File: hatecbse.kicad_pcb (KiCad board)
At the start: 2 copper layers, 79 x 88.8 mm, 20 parts, among them J1 Screw_Terminal_01x06, J2 Screw_Terminal_01x06, J3 Barrel_Jack_MountingPin, J4 Conn_01x04_Socket, J5 Conn_01x03, J6 Conn_01x02_Pin, J7 Conn_01x02_Pin, J8 Conn_01x04_Pin, U1 TMC2209_SILENTSTEPSTICK, U2 TMC2209_SILENTSTEPSTICK

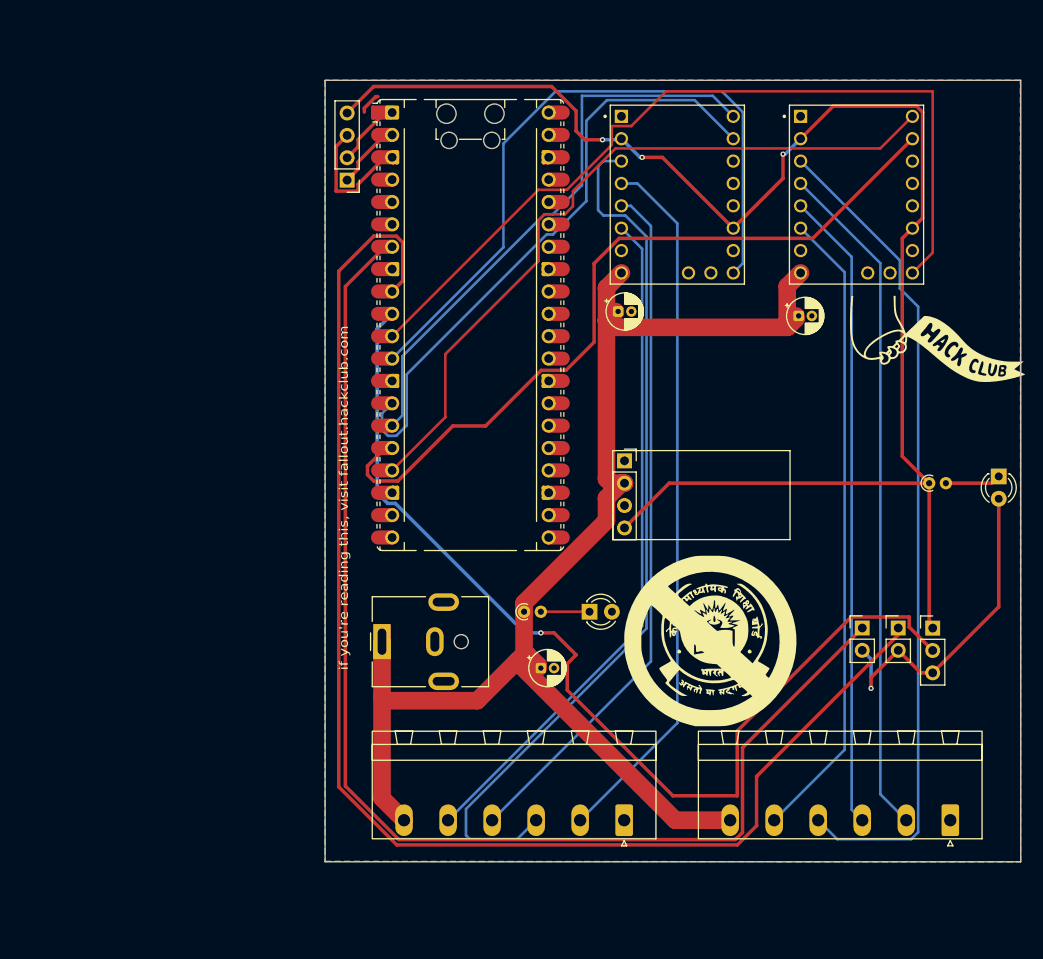
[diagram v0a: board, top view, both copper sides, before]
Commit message: diddy
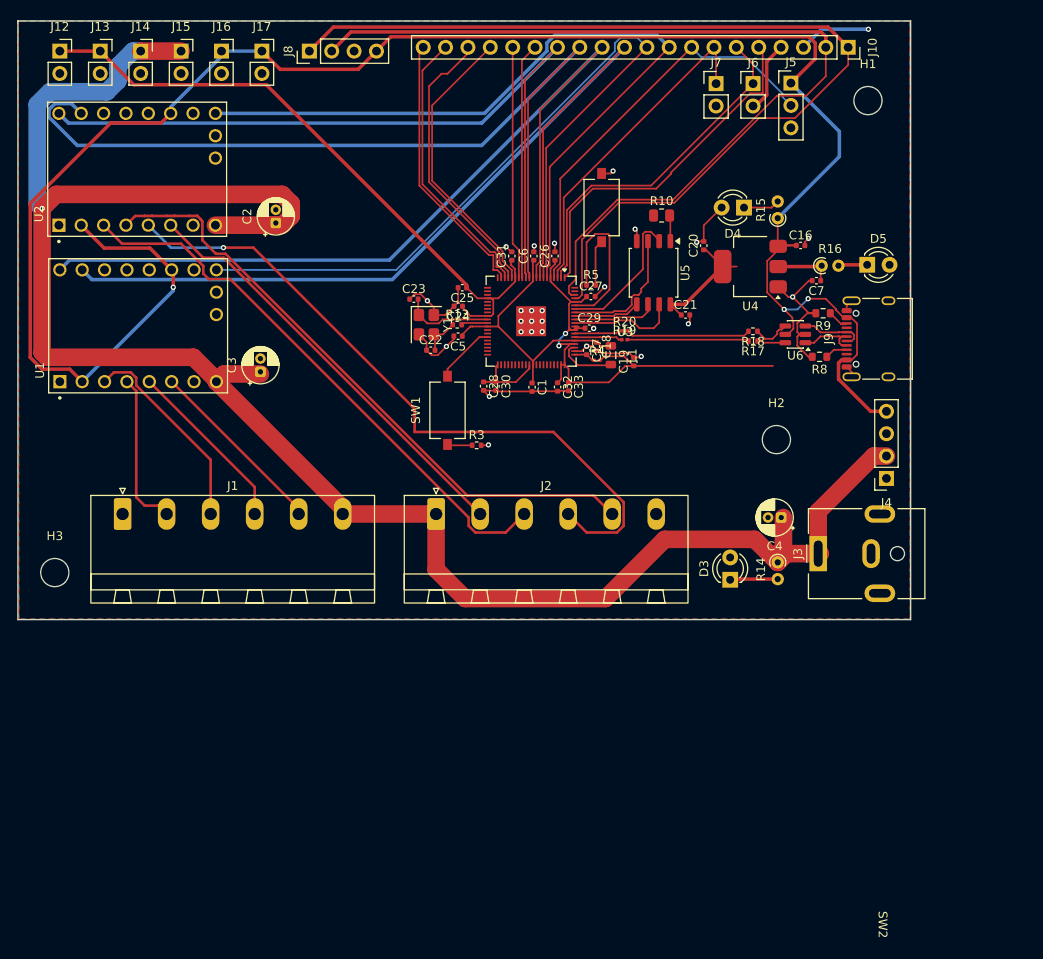
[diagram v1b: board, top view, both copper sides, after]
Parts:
- removed A1: RaspberryPi_Pico, Module:RaspberryPi_Pico_Common_Unspecified
- removed D1, D2: LED, LED_THT:LED_D3.0mm
- removed G*** (x2): LOGO, LOGO
- removed R1: 1.2k, Resistor_THT:R_Axial_DIN0204_L3.6mm_D1.6mm_P1.90mm_Vertical
- removed R2: 500, Resistor_THT:R_Axial_DIN0204_L3.6mm_D1.6mm_P1.90mm_Vertical
- added C1: 100 n, Capacitor_SMD:C_0402_1005Metric, F.Cu at (131.5, 94.6)
- added C16: 10 u, Capacitor_SMD:C_0402_1005Metric, F.Cu at (162.0, 78.5)
- added C17: 4.7 u, Capacitor_SMD:C_0402_1005Metric, F.Cu at (137.7, 90.4)
- added C18: 4.7 u, Capacitor_SMD:C_0402_1005Metric, F.Cu at (138.8, 90.0)
- added C19: 4.7 u, Capacitor_SMD:C_0402_1005Metric, F.Cu at (143.1, 91.7)
- added C20: 10 u, Capacitor_SMD:C_0402_1005Metric, F.Cu at (151.0, 78.5)
- added C21: 100 n, Capacitor_SMD:C_0402_1005Metric, F.Cu at (148.9, 86.4)
- added C22: 15 p, Capacitor_SMD:C_0402_1005Metric, F.Cu at (120.0, 90.4)
- added C23: 15 p, Capacitor_SMD:C_0402_1005Metric, F.Cu at (118.1, 84.6)
- added C24: 100 n, Capacitor_SMD:C_0402_1005Metric, F.Cu at (123.1, 85.4)
- added C25: 100 n, Capacitor_SMD:C_0402_1005Metric, F.Cu at (123.6, 83.3)
- added C26: 100 n, Capacitor_SMD:C_0402_1005Metric, F.Cu at (134.1, 79.7)
- added C27: 100 n, Capacitor_SMD:C_0402_1005Metric, F.Cu at (138.2, 84.3)
- added C28: 100 n, Capacitor_SMD:C_0402_1005Metric, F.Cu at (126.0, 94.5)
- added C29: 100 n, Capacitor_SMD:C_0402_1005Metric, F.Cu at (138.0, 87.9)
- added C30: 100 n, Capacitor_SMD:C_0402_1005Metric, F.Cu at (127.4, 94.5)
- added C31: 100 n, Capacitor_SMD:C_0402_1005Metric, F.Cu at (129.2, 79.7)
- added C32: 100 n, Capacitor_SMD:C_0402_1005Metric, F.Cu at (134.4, 94.6)
- added C33: 100 n, Capacitor_SMD:C_0402_1005Metric, F.Cu at (135.7, 94.5)
- added C5: 4.7 u, Capacitor_SMD:C_0402_1005Metric, F.Cu at (123.1, 88.8)
- added C6: 100 n, Capacitor_SMD:C_0402_1005Metric, F.Cu at (131.7, 79.7)
- added C7: 10 uF, Capacitor_SMD:C_0402_1005Metric, F.Cu at (163.8, 82.5)
- added D3: LED, LED_THT:LED_D3.0mm, F.Cu at (154.0, 116.5)
- added D4: LED, LED_THT:LED_D3.0mm, F.Cu at (155.6, 74.2)
- added D5: LED, LED_THT:LED_D3.0mm, F.Cu at (169.6, 80.7)
- added H1: MountingHole, MountingHole:MountingHole_3.2mm_M3, F.Cu at (169.7, 62.0)
- added H2: MountingHole, MountingHole:MountingHole_3.2mm_M3, F.Cu at (159.2, 100.5)
- added H3: MountingHole, MountingHole:MountingHole_3.2mm_M3, F.Cu at (77.3, 115.7)
- added J10: Conn_01x20_Pin, Connector_PinSocket_2.54mm:PinSocket_1x20_P2.54mm_Vertical, F.Cu at (167.4, 56.0)
- added J12: Conn_01x02_Pin, Connector_PinSocket_2.54mm:PinSocket_1x02_P2.54mm_Vertical, F.Cu at (77.9, 56.4)
- added J13: Conn_01x02_Pin, Connector_PinSocket_2.54mm:PinSocket_1x02_P2.54mm_Vertical, F.Cu at (82.5, 56.4)
- added J14: Conn_01x02_Pin, Connector_PinSocket_2.54mm:PinSocket_1x02_P2.54mm_Vertical, F.Cu at (87.0, 56.4)
- added J15: Conn_01x02_Pin, Connector_PinSocket_2.54mm:PinSocket_1x02_P2.54mm_Vertical, F.Cu at (91.6, 56.4)
- added J16: Conn_01x02_Pin, Connector_PinSocket_2.54mm:PinSocket_1x02_P2.54mm_Vertical, F.Cu at (96.2, 56.4)
- added J17: Conn_01x02_Pin, Connector_PinSocket_2.54mm:PinSocket_1x02_P2.54mm_Vertical, F.Cu at (100.8, 56.4)
- added J9: USB_C_Receptacle_USB2.0_14P, Connector_USB:USB_C_Receptacle_XKB_U262-16XN-4BVC11, F.Cu at (170.9, 89.1)
- added L1: 3.3 u, Inductor_SMD:L_0805_2012Metric, F.Cu at (140.4, 91.0)
- added R10: 0, Resistor_SMD:R_0805_2012Metric, F.Cu at (146.2, 75.1)
- added R13: 1k, Resistor_SMD:R_0402_1005Metric, F.Cu at (123.0, 87.5)
- added R14: 1.2k, Resistor_THT:R_Axial_DIN0204_L3.6mm_D1.6mm_P1.90mm_Vertical, F.Cu at (159.4, 114.5)
- added R15: 500, Resistor_THT:R_Axial_DIN0204_L3.6mm_D1.6mm_P1.90mm_Vertical, F.Cu at (159.4, 75.4)
- added R16: 330, Resistor_THT:R_Axial_DIN0204_L3.6mm_D1.6mm_P1.90mm_Vertical, F.Cu at (164.4, 80.8)
- added R17: 33R, Resistor_SMD:R_0402_1005Metric, F.Cu at (156.6, 89.3)
- added R18: 33R, Resistor_SMD:R_0402_1005Metric, F.Cu at (156.6, 88.2)
- added R19: 27, Resistor_SMD:R_0201_0603Metric, F.Cu at (142.0, 89.2)
- added R20: 27, Resistor_SMD:R_0201_0603Metric, F.Cu at (142.0, 88.2)
- added R3: 1k, Resistor_SMD:R_0402_1005Metric, F.Cu at (125.2, 101.2)
- added R4: 33, Resistor_SMD:R_0201_0603Metric, F.Cu at (138.9, 91.5)
- added R5: 1k, Resistor_SMD:R_0402_1005Metric, F.Cu at (138.2, 83.0)
- added R8: 5.1k, Resistor_SMD:R_0603_1608Metric, F.Cu at (164.2, 91.2)
- added R9: 5.1k, Resistor_SMD:R_0603_1608Metric, F.Cu at (164.6, 86.2)
- added SW1: SW_Push, Button_Switch_SMD:SW_Tactile_SPST_NO_Straight_CK_PTS636Sx25SMTRLFS, F.Cu at (121.9, 97.2)
- added SW2: SW_Push, Button_Switch_SMD:SW_Tactile_SPST_NO_Straight_CK_PTS636Sx25SMTRLFS, F.Cu at (139.4, 74.2)
- added U3: RP2350B, Package_DFN_QFN:QFN-80-1EP_10x10mm_P0.4mm_EP3.4x3.4mm, F.Cu at (131.4, 87.1)
- added U4: NCP1117-3.3_SOT223, Package_TO_SOT_SMD:SOT-223-3_TabPin2, F.Cu at (156.3, 80.9)
- added U5: W25Q128JVS, Package_SO:SOIC-8_5.3x5.3mm_P1.27mm, F.Cu at (145.3, 81.6)
- added U6: USBLC6-2SC6, Package_TO_SOT_SMD:SOT-23-6, F.Cu at (161.4, 88.6)
- added Y1: Crystal_GND24, Crystal:Crystal_SMD_Abracon_ABM8G-4Pin_3.2x2.5mm, F.Cu at (119.5, 87.5)
- moved U2 81.8 mm to (86.7, 69.8), turned to 90 degrees
- moved J2 68.0 mm to (120.6, 109.0), turned to 0 degrees
- moved J1 66.7 mm to (85.0, 109.0), turned to 0 degrees
- moved J7 65.2 mm to (152.4, 60.1)
- moved J5 64.0 mm to (160.9, 60.1)
- moved J6 63.1 mm to (156.6, 60.1)
- moved U1 63.0 mm to (86.8, 87.6), turned to 90 degrees
- moved C2 60.3 mm to (102.4, 76.0), turned to 90 degrees
- moved J3 50.5 mm to (164.0, 113.5)
- moved C3 41.2 mm to (100.7, 92.8), turned to 90 degrees
- moved C4 32.2 mm to (159.8, 109.4), turned to 180 degrees
- moved J4 29.8 mm to (171.8, 105.0), turned to 180 degrees
- moved J8 15.3 mm to (106.2, 56.4), turned to 90 degrees
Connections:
- J2 pad 1: GND -> +12V
- J2 pad 2: M2_1A -> M2_2B
- J2 pad 3: M2_2A -> M2_1B
- J2 pad 4: M2_1B -> M2_2A
- J2 pad 5: M2_2B -> M2_1A
- J2 pad 6: +12V -> GND
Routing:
- net VREG_VIN: track 0.00 -> 165.7 mm, vias 0 -> 3
- net LS_2: track 154.1 -> 37.7 mm
- net SCL: track 7.72 -> 111.0 mm
- net LS_1: track 139.9 -> 39.9 mm
- net SDA: track 7.72 -> 104.8 mm
- net M1_1B: track 100.2 -> 23.3 mm
- net SERVO: track 117.1 -> 48.0 mm, vias 1 -> 0
- net +12V: track 155.5 -> 223.2 mm, vias 0 -> 1
- net M1_1A: track 80.6 -> 17.8 mm
- net M1_2A: track 79.3 -> 20.0 mm
- net M1_2B: track 77.3 -> 21.0 mm
- net +5V: track 180.4 -> 224.3 mm
- net GPIO4: track 0.00 -> 40.7 mm
- net DIR_1: track 65.1 -> 101.3 mm
- net STEP_1: track 70.0 -> 103.5 mm
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- added copper zone on In2.Cu, net GND
- added copper zone on F.Cu, net VREG_VIN
- removed copper zone on F.Cu, net GND
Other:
- board size 79 x 88.8 mm -> 101.4 x 68 mm
- copper layers 2 -> 4
- board text removed: "if you're reading this, visit fallout.hackclub.com"
